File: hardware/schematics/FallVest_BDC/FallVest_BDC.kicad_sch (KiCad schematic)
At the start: 7 parts, among them Q1 AO3400A, U1 ICM-20948, U2 ESP32-WROOM-32, U3 4554, U4 NEO-6M

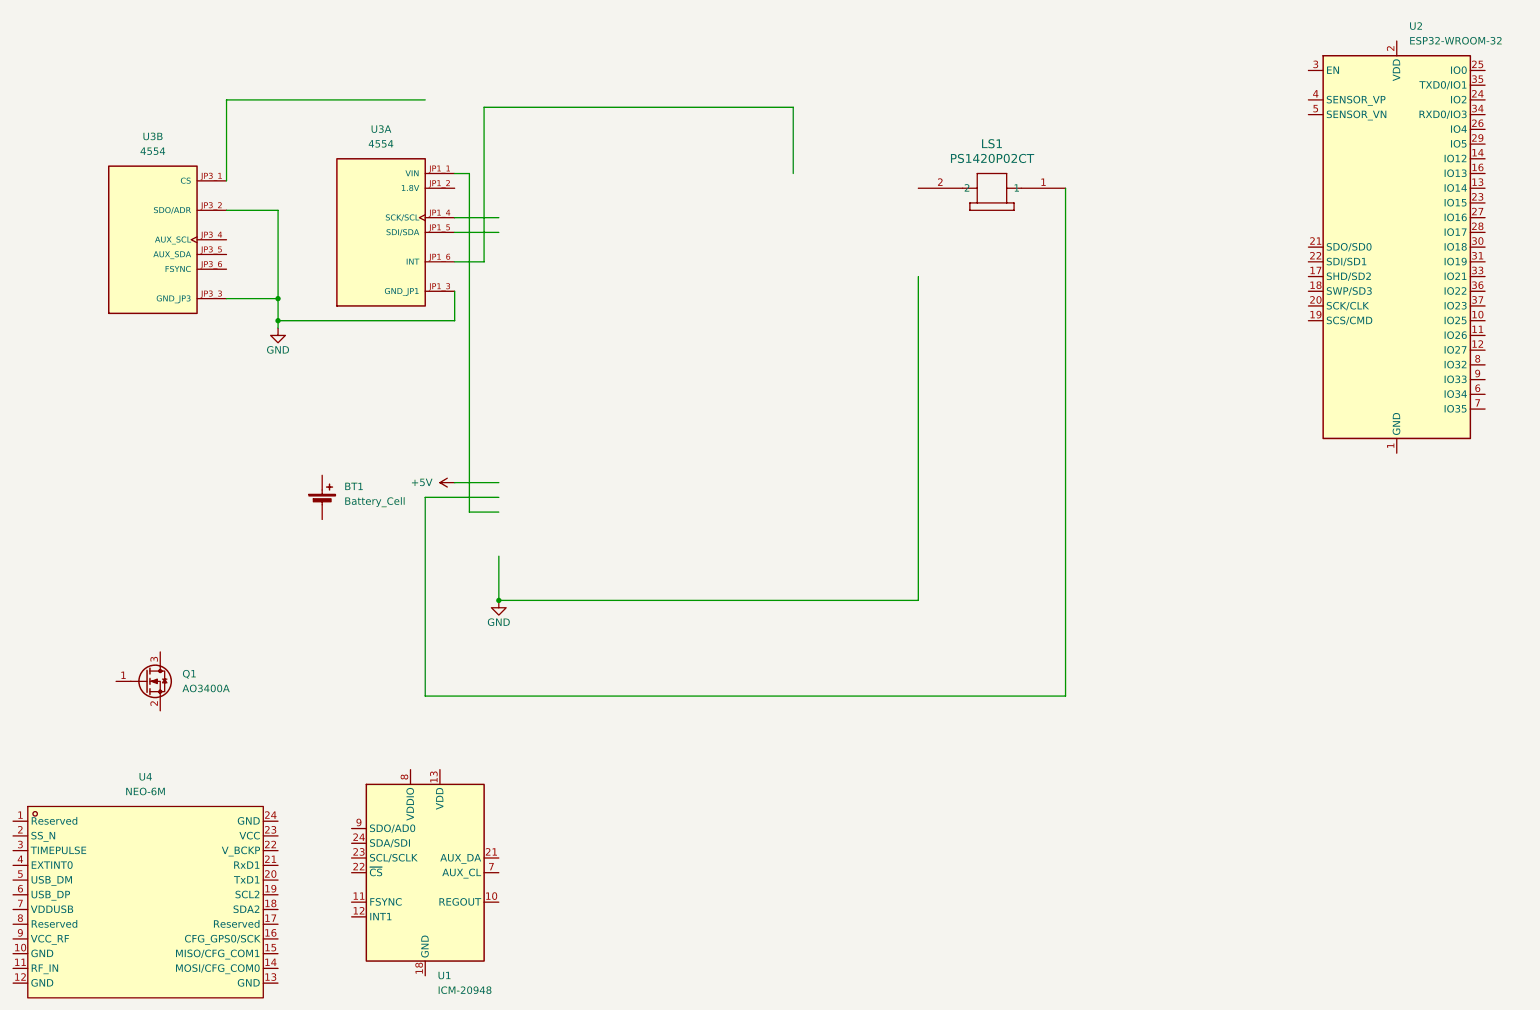
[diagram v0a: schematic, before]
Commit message: Update
Some minor tweaking.
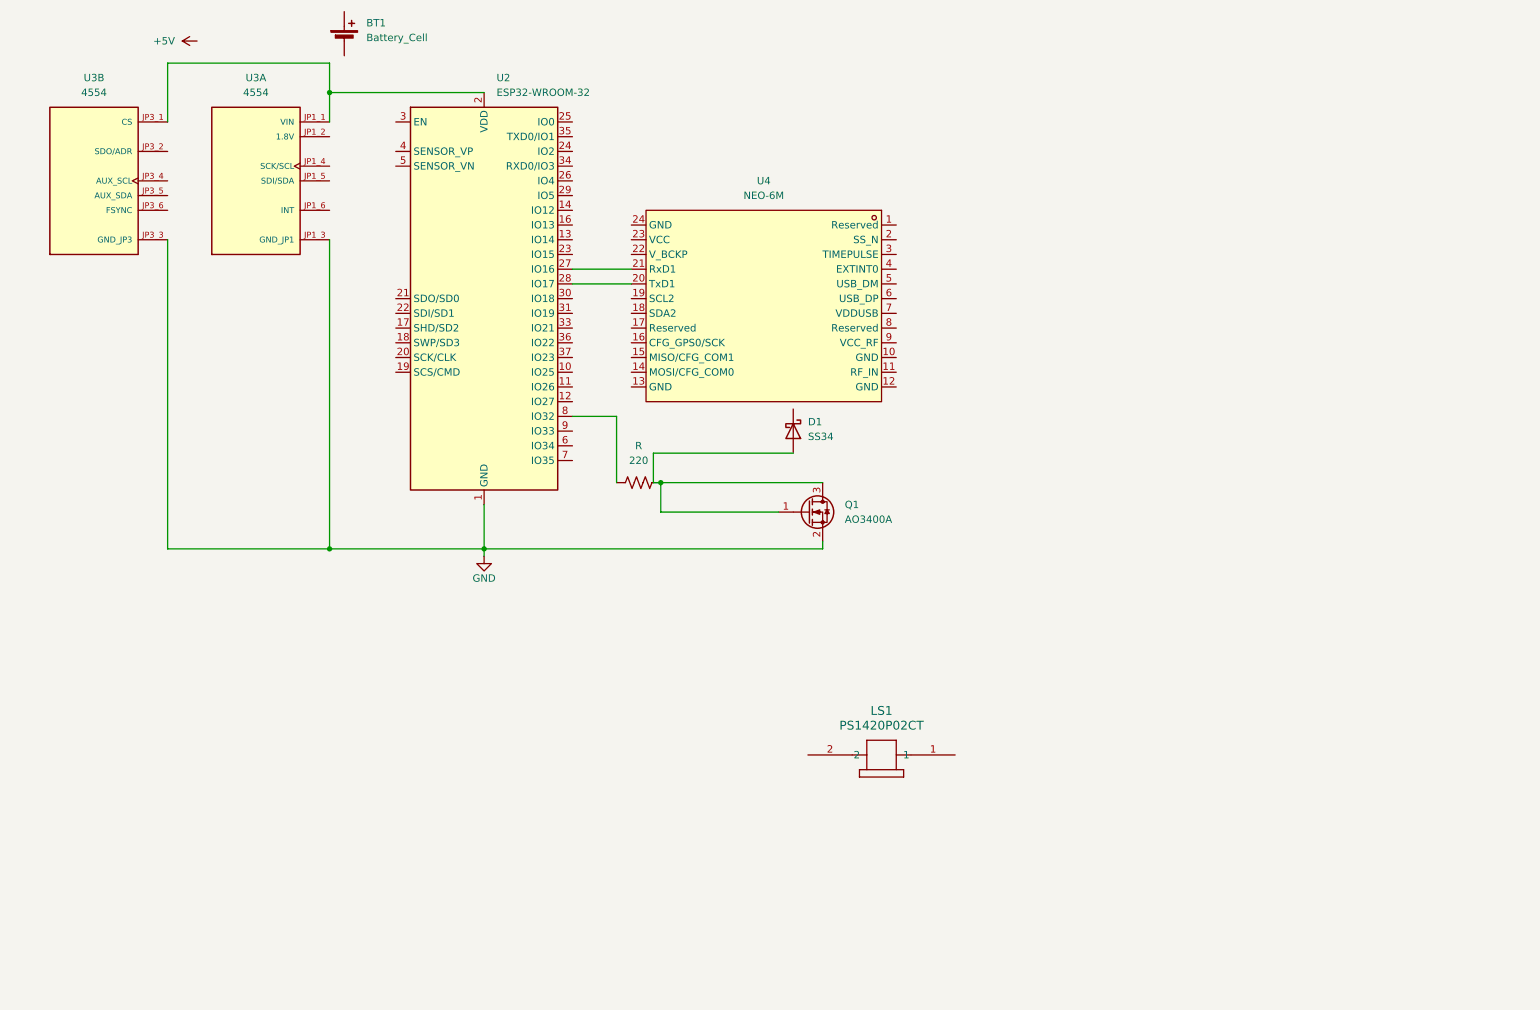
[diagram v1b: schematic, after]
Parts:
- removed U1: ICM-20948, Sensor_Motion:InvenSense_QFN-24_3x3mm_P0.4mm, symbol Sensor_Motion:ICM-20948
- added D1: SS34, Diode_SMD:D_SMA, symbol Diode:SS34
- added R: 220, symbol Device:R_US
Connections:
- net GND: now also Q1.2 (S), U2.1 (GND), U2.15 (GND), U2.38 (GND), U2.39 (GND); no longer U3.JP3_2 (SDO/ADR)
- net at Q1.1 (G): now also Q1.3 (D), D1.2 (A), R.2
- net at U4.20 (TxD1): now also U2.28 (IO17)
- net at U4.21 (RxD1): now also U2.27 (IO16)
- net at U3.JP3_1 (CS): now also U2.2 (VDD), U3.JP1_1 (VIN)
- net at U2.8 (IO32): now also R.1
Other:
- moved on the sheet: BT1, LS1, Q1, U2, U3A, U3B, U4
